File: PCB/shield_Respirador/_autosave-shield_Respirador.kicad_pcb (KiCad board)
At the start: 2 copper layers, 137.3 x 102 mm, 31 parts, among them P1 Digital, P10 CONN_01X01, P11 CONN_01X01, P12 CONN_01X01, P13 CONN_01X01, P2 Power, P3 Analog, P4 Analog, P5 PWM, P6 PWM, P7 Communication, P8 CONN_01X01, P9 CONN_01X01

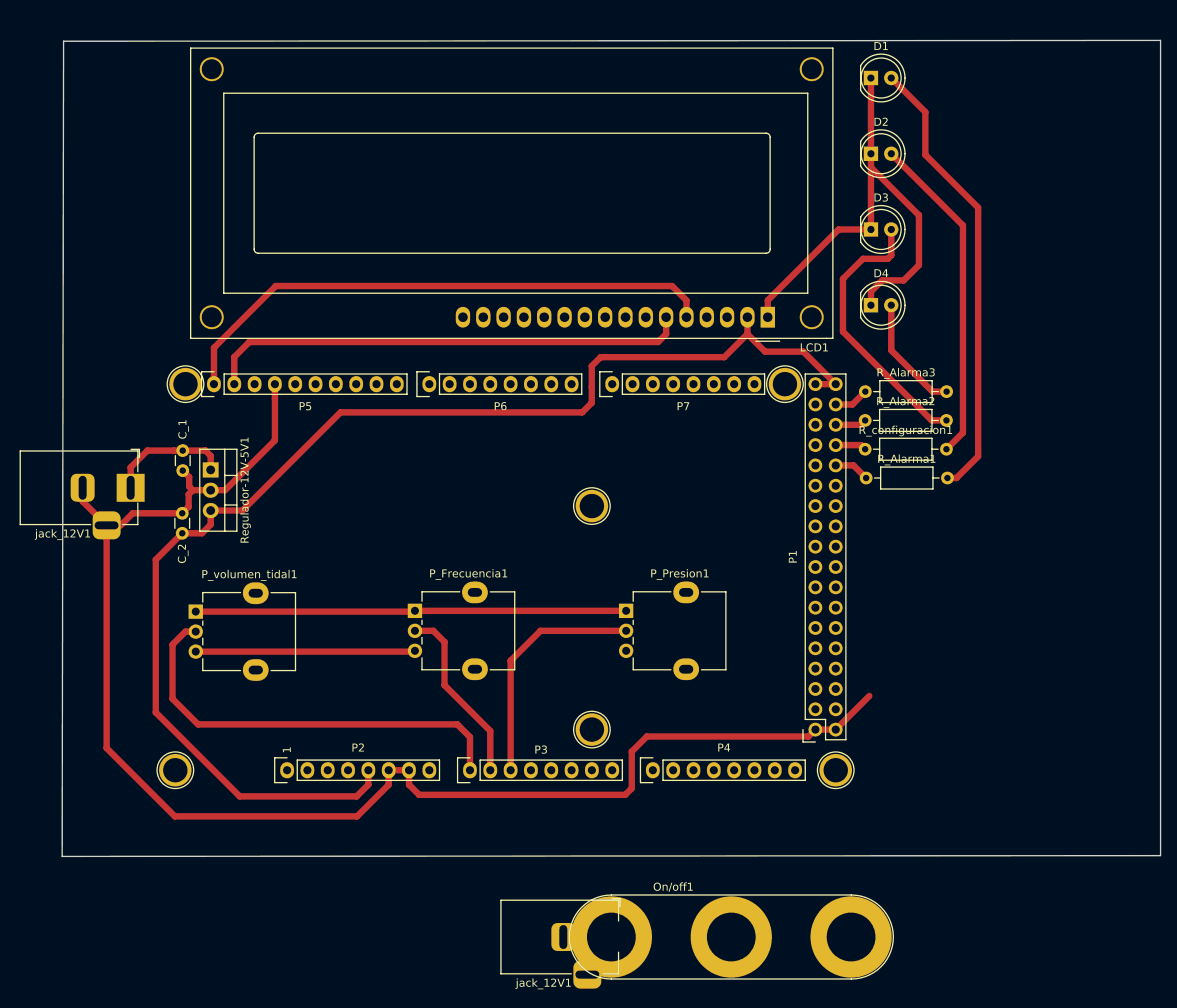
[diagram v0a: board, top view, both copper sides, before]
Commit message: version 0.4
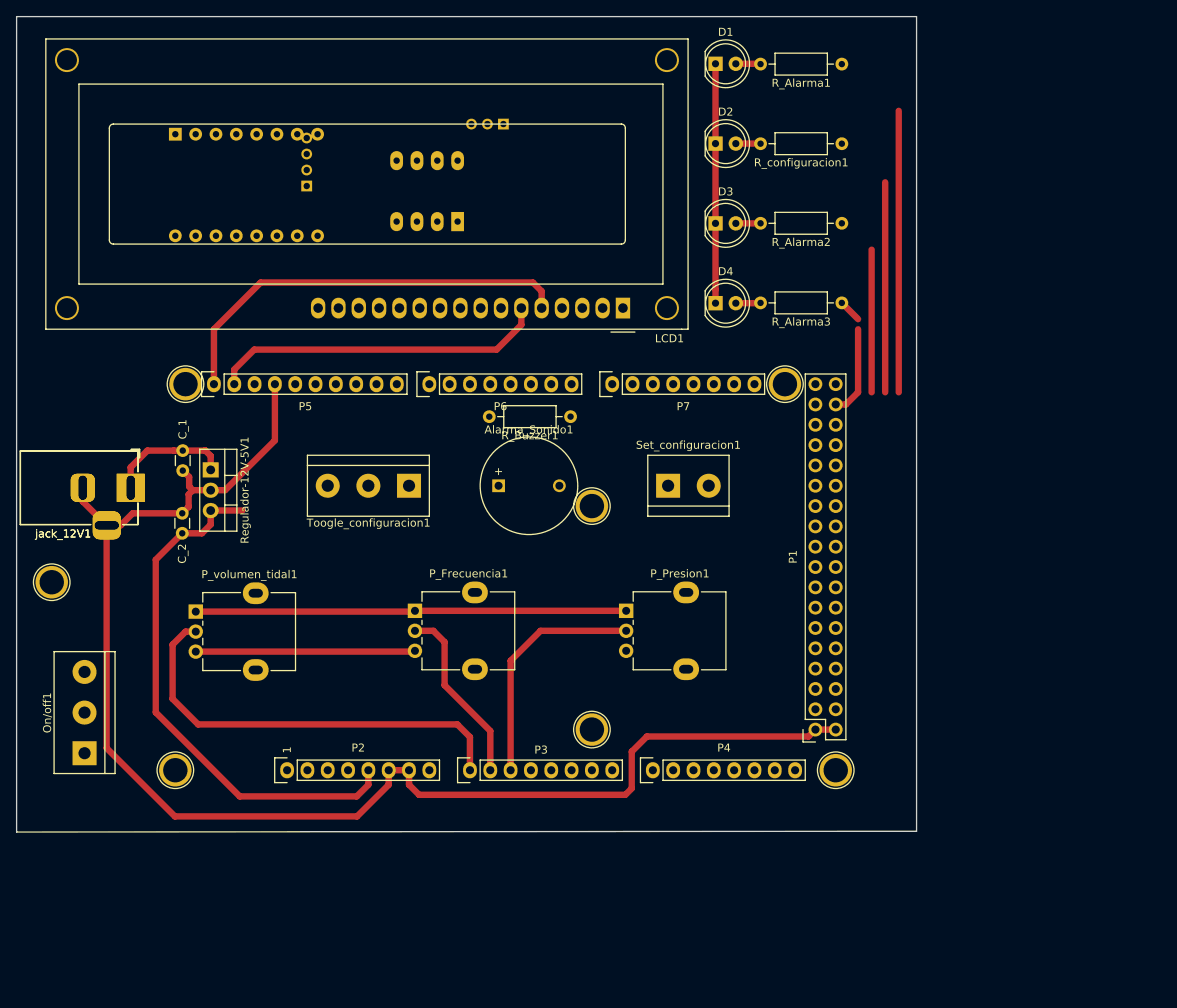
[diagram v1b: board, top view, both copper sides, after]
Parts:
- added Alarma_Sonido1: Buzzer, Buzzer_Beeper:MagneticBuzzer_ProSignal_ABI-009-RC, F.Cu at (157.8, 83.6)
- added Drivermotor1: Pololu_Breakout_DRV8825, Module:Pololu_Breakout-16_15.2x20.3mm, B.Cu at (117.3, 39.6)
- added Final_De_Carrera1: Conn_01x03_Female, Connector_PinSocket_2.00mm:PinSocket_1x03_P2.00mm_Vertical, B.Cu at (158.4, 38.4)
- added P10: CONN_01X01, Socket_Arduino_Mega:Arduino_1pin, F.Cu at (101.9, 95.6)
- added R_Buzzer1: 220, Resistor_THT:R_Axial_DIN0207_L6.3mm_D2.5mm_P10.16mm_Horizontal, F.Cu at (166.8, 74.9)
- added Sensor_Presion1: MPXA6115A, Package_DIP:DIP-8_W7.62mm_LongPads, B.Cu at (152.6, 50.5)
- added Set_configuracion1: SW_Push, TerminalBlock:TerminalBlock_bornier-2_P5.08mm, F.Cu at (178.9, 83.6)
- added Toogle_configuracion1: SW_Push_SPDT, TerminalBlock:TerminalBlock_bornier-3_P5.08mm, F.Cu at (146.6, 83.6)
- added conector_motor1: Conn_01x04_Female, Connector_PinSocket_2.00mm:PinSocket_1x04_P2.00mm_Vertical, B.Cu at (133.8, 46.1)
- On/off1: footprint Connector:Banana_Jack_3Pin -> TerminalBlock:TerminalBlock_bornier-3_P5.08mm
- moved jack_12V1 82.2 mm to (111.8, 83.8)
- moved On/off1 69.7 mm to (106.0, 117.0), turned to 90 degrees
- moved R_Alarma1 51.8 mm to (200.7, 30.9), turned to 180 degrees
- moved R_configuracion1 38.3 mm to (200.7, 40.8), turned to 180 degrees
- moved R_Alarma2 24.8 mm to (200.7, 50.8), turned to 180 degrees
- moved D1 19.5 mm to (184.9, 30.8)
- moved D2 19.5 mm to (184.9, 40.8)
- moved D3 19.4 mm to (184.9, 50.8)
- moved D4 19.4 mm to (184.9, 60.7)
- moved LCD1 18.1 mm to (173.3, 61.4)
- moved R_Alarma3 11.5 mm to (200.7, 60.7), turned to 180 degrees
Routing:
- net +5V: track 160.1 -> 66.8 mm
- net Net-(D1-Pad2): track 56.8 -> 3.11 mm
- net Net-(D2-Pad2): track 41.5 -> 3.10 mm
- net GND: track 244.0 -> 206.6 mm
- net Net-(D3-Pad2): track 34.6 -> 3.10 mm
- net /29: track 4.45 -> 35.2 mm
- net /27: track 3.89 -> 26.2 mm
- net /SDA: track 60.7 -> 42.1 mm
- net /SCL: track 69.7 -> 52.8 mm
- net /25: track 3.90 -> 17.8 mm
- net Net-(D4-Pad2): track 14.7 -> 3.11 mm
- net /23: track 4.37 -> 14.2 mm
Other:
- board size 137.3 x 102 mm -> 112.5 x 101.9 mm
